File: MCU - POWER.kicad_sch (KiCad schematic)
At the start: 22 parts, among them U1 STM32G474RET6, U2 STM32G474RET6

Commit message: [01/07/2026][MCU - IOs] Update
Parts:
- U1, U2: footprint (none) -> Duc_Library:LQFP-64_L10.0-W10.0-P0.50-LS12.0-BL; private Datasheet -> (none)
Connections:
- new net: C7., C9., FB1., U1.28 (VREF+), U1.29 (VDDA)
- new net: C14., C18., FB2., U2.28 (VREF+), U2.29 (VDDA)
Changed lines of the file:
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@@
 	(title_block
 		(title "MCU - POWER")
-		(date "2025-01-12")
+		(date "2026-06-27")
 		(rev "${REVISION}")
 		(company "${COMPANY}")
@@
 	)
 	(symbol
+		(lib_name "PBBHAQ2012H-102T10_1")
 		(lib_id "Duc_Library:PBBHAQ2012H-102T10")
 		(at 147.32 78.74 0)
@@
 	)
 	(symbol
-		(lib_name "PBBHAQ2012H-102T10_1")
 		(lib_id "Duc_Library:PBBHAQ2012H-102T10")
 		(at 147.32 144.78 0)
@@
 			)
 		)
-		(property private "Footprint" "Duc_Library:LQFP-64_L10.0-W10.0-P0.50-LS12.0-BL"
+		(property "Footprint" "Duc_Library:LQFP-64_L10.0-W10.0-P0.50-LS12.0-BL"
 			(at 225.552 98.044 0)
 			(effects
@@
 			)
 		)
-		(property private "Datasheet" "https://lcsc.com/product-detail/No-specification-for-star-making-plan_STMicroelectronics-STM32G474RET6_C521608.html"
+		(property "Datasheet" "https://lcsc.com/product-detail/No-specification-for-star-making-plan_STMicroelectronics-STM32G474RET6_C521608.html"
 			(at 233.68 100.33 0)
 			(do_not_autoplace yes)
@@
 			)
 		)
-		(property private "Footprint" "Duc_Library:LQFP-64_L10.0-W10.0-P0.50-LS12.0-BL"
+		(property "Footprint" "Duc_Library:LQFP-64_L10.0-W10.0-P0.50-LS12.0-BL"
 			(at 225.552 164.084 0)
 			(effects
@@
 			)
 		)
-		(property private "Datasheet" "https://lcsc.com/product-detail/No-specification-for-star-making-plan_STMicroelectronics-STM32G474RET6_C521608.html"
+		(property "Datasheet" "https://lcsc.com/product-detail/No-specification-for-star-making-plan_STMicroelectronics-STM32G474RET6_C521608.html"
 			(at 233.68 166.37 0)
 			(do_not_autoplace yes)
@@
 	)
 	(symbol
-		(lib_name "CC0402KRX7R6BB105_3")
+		(lib_name "CC0402KRX7R6BB105_5")
 		(lib_id "Duc_Library:CC0402KRX7R6BB105")
 		(at 182.88 114.3 90)
@@
 	)
 	(symbol
-		(lib_name "CC0402KRX7R9BB104_3")
+		(lib_name "CC0402KRX7R9BB104_2")
 		(lib_id "Duc_Library:CC0402KRX7R9BB104")
 		(at 182.88 152.4 90)
@@
 	)
 	(symbol
-		(lib_name "CC0402KRX7R9BB104_9")
+		(lib_name "CC0402KRX7R9BB104_8")
 		(lib_id "Duc_Library:CC0402KRX7R9BB104")
 		(at 182.88 86.36 90)
@@
 	)
 	(symbol
-		(lib_name "CC0402KRX7R9BB104_2")
+		(lib_name "CC0402KRX7R9BB104_4")
 		(lib_id "Duc_Library:CC0402KRX7R9BB104")
 		(at 182.88 134.62 90)
@@
 	)
 	(symbol
-		(lib_name "CC0402KRX7R9BB104_8")
+		(lib_name "CC0402KRX7R9BB104_7")
 		(lib_id "Duc_Library:CC0402KRX7R9BB104")
 		(at 162.56 134.62 90)
@@
 	)
 	(symbol
-		(lib_name "CC0402KRX7R9BB104_4")
+		(lib_name "CC0402KRX7R9BB104_9")
 		(lib_id "Duc_Library:CC0402KRX7R9BB104")
 		(at 162.56 68.58 90)
@@
 	)
 	(symbol
-		(lib_name "CC0402KRX7R9BB104_5")
+		(lib_name "CC0402KRX7R9BB104_3")
 		(lib_id "Duc_Library:CC0402KRX7R9BB104")
 		(at 139.7 68.58 90)
@@
 	)
 	(symbol
-		(lib_name "CC0402KRX7R6BB105_5")
+		(lib_name "CC0402KRX7R6BB105_3")
 		(lib_id "Duc_Library:CC0402KRX7R6BB105")
 		(at 160.02 152.4 90)
@@
 	)
 	(symbol
-		(lib_name "CC0402KRX7R9BB104_6")
+		(lib_name "CC0402KRX7R9BB104_5")
 		(lib_id "Duc_Library:CC0402KRX7R9BB104")
 		(at 182.88 68.58 90)
@@
 	)
 	(symbol
-		(lib_name "CC0402KRX7R9BB104_7")
+		(lib_name "CC0402KRX7R9BB104_6")
 		(lib_id "Duc_Library:CC0402KRX7R9BB104")
 		(at 116.84 134.62 90)

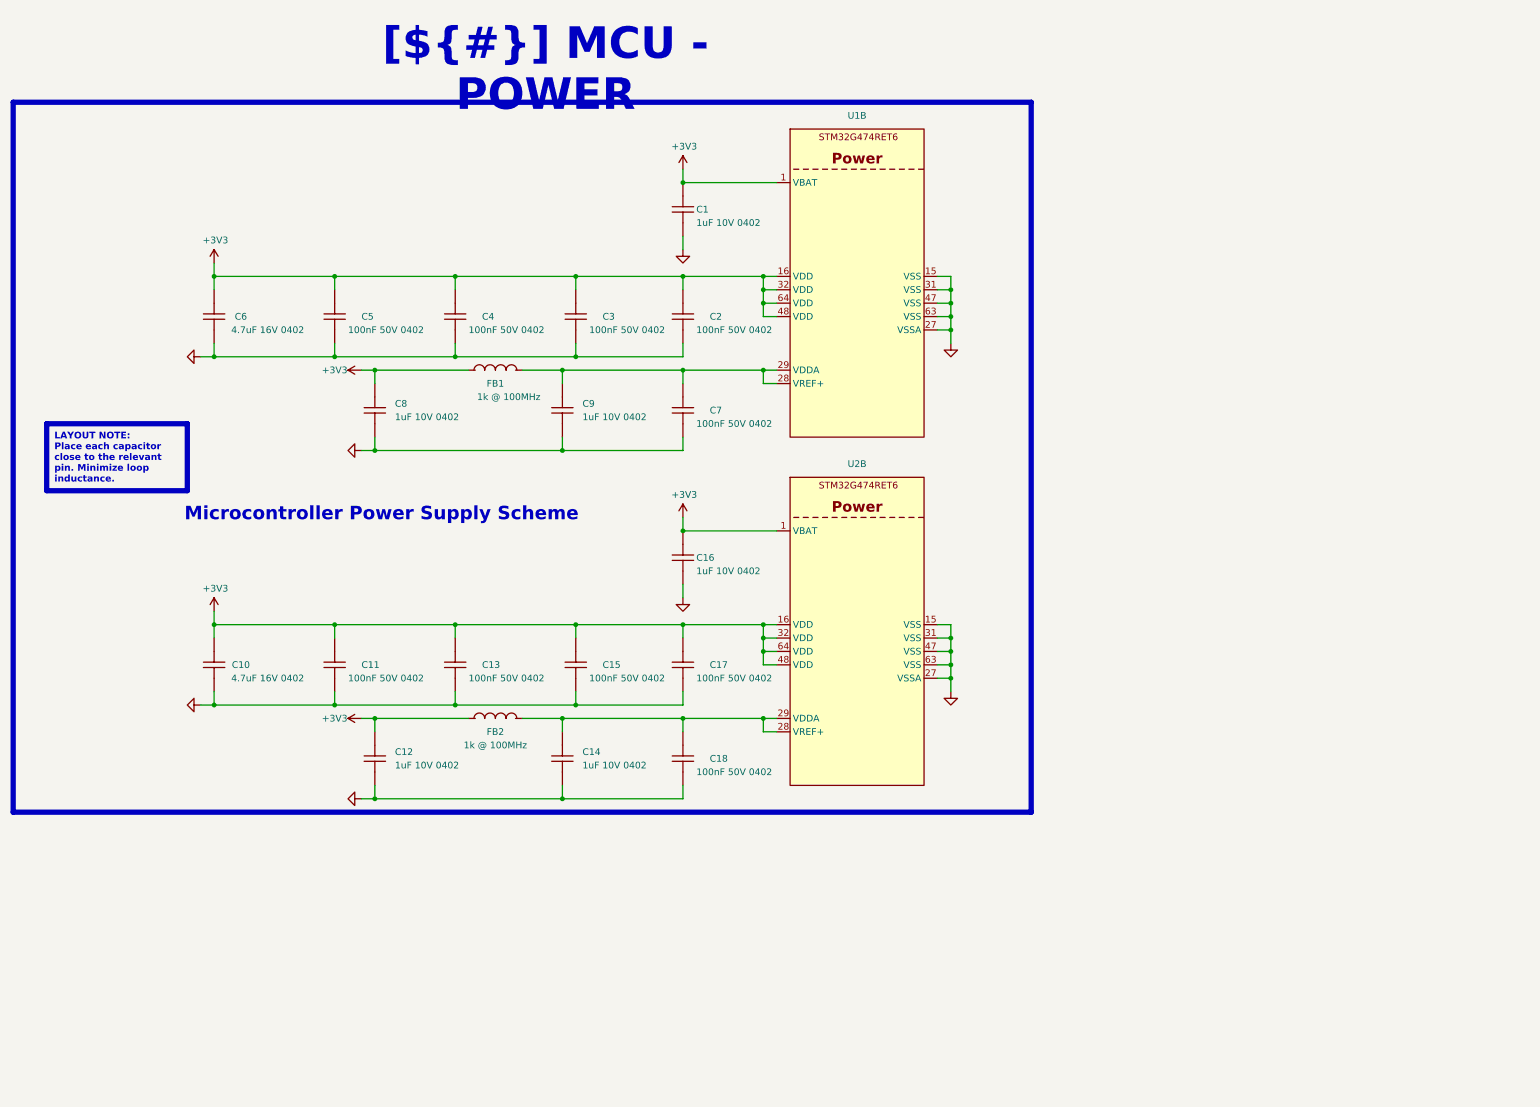
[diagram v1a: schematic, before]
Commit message: Update Power Generation Schematic
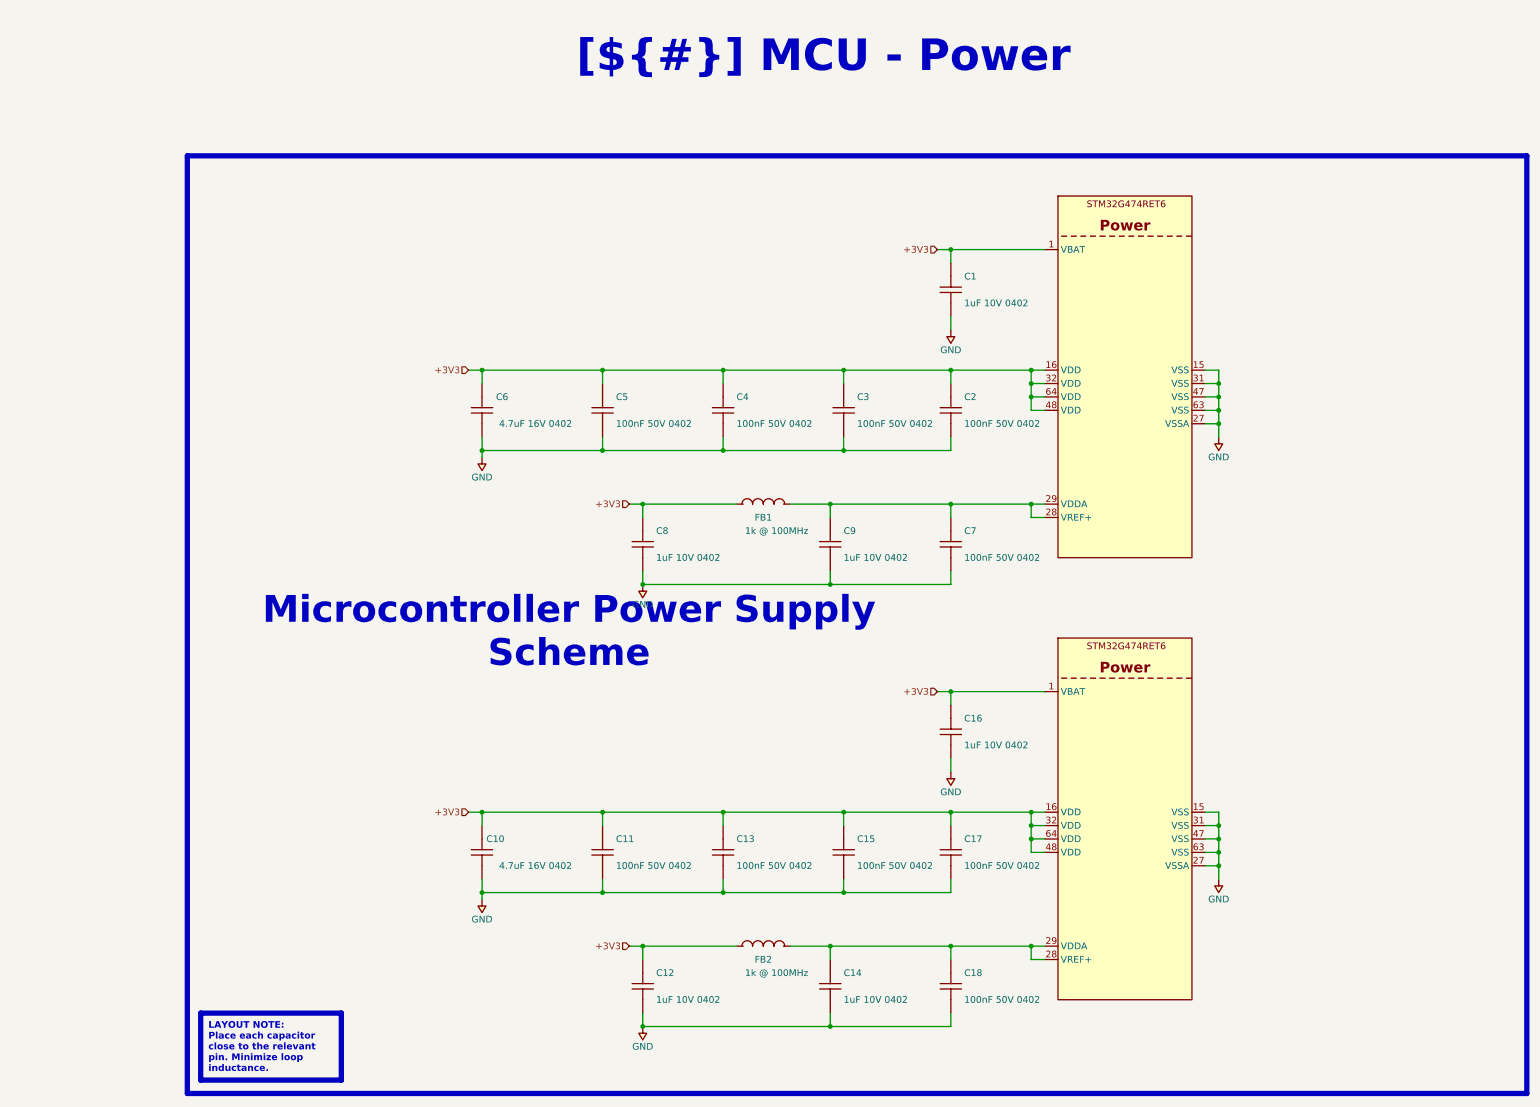
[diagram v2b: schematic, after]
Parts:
- removed U1, U2: STM32G474RET6, Duc_Library:LQFP-64_L10.0-W10.0-P0.50-LS12.0-BL, symbol Duc_Library:STM32G474RET6
- added U1, U2: STM32G474RET6, Duc_Library:LQFP-64_L10.0-W10.0-P0.50-LS12.0-BL, symbol Duc-MCUs:STM32G474RET6
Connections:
- net +3V3: now also U1.1 (VBAT), U1.16 (VDD), U1.32 (VDD), U1.48 (VDD), U1.64 (VDD), U2.1 (VBAT), U2.16 (VDD), U2.32 (VDD), U2.48 (VDD), U2.64 (VDD)
- net GND: now also U1.15 (VSS), U1.27 (VSSA), U1.31 (VSS), U1.47 (VSS), U1.63 (VSS), U2.15 (VSS), U2.27 (VSSA), U2.31 (VSS), U2.47 (VSS), U2.63 (VSS)
- new net: C7., C9., FB1., U1.28 (VREF+), U1.29 (VDDA)
- new net: C14., C18., FB2., U2.28 (VREF+), U2.29 (VDDA)
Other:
- title: MCU - POWER -> MCU - Power
- moved on the sheet: C1, C2, C3, C4, C5, C6, C7, C8, C9, FB1
